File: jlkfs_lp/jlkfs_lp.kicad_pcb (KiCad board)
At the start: 2 copper layers, 139 x 121.8 mm, 38 parts, among them J0 USB_C_Receptacle_PowerOnly_6P, SW0 SWITCH, SW1 SWITCH, SW10 SWITCH, SW11 SWITCH, SW12 SWITCH, SW13 SWITCH, SW14 SWITCH, SW15 SWITCH, SW16 SWITCH, SW17 SWITCH, SW18 SWITCH, SW19 SWITCH, SW2 SWITCH, SW20 SWITCH, SW21 SWITCH, SW22 SWITCH, SW23 SWITCH, SW24 SWITCH, SW25 SWITCH, SW26 SWITCH, SW27 SWITCH, SW28 SWITCH, SW3 SWITCH, SW4 SWITCH, SW5 SWITCH, SW6 SWITCH, SW7 SWITCH, SW8 SWITCH, SW9 SWITCH, U0 RP2040

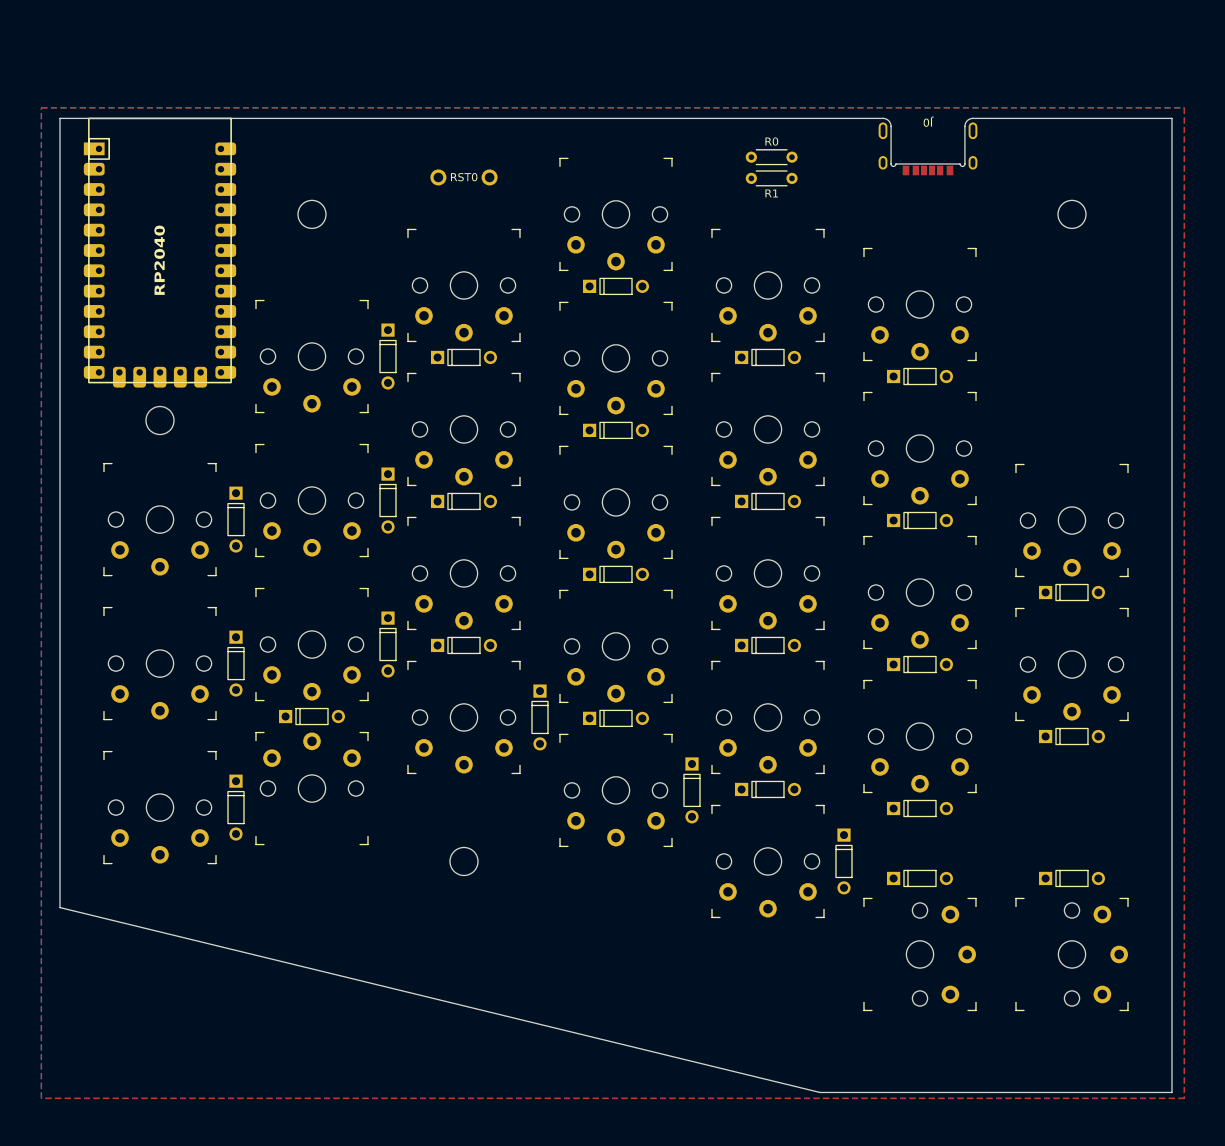
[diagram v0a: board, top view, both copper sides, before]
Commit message: Updates to jlkfs_lp
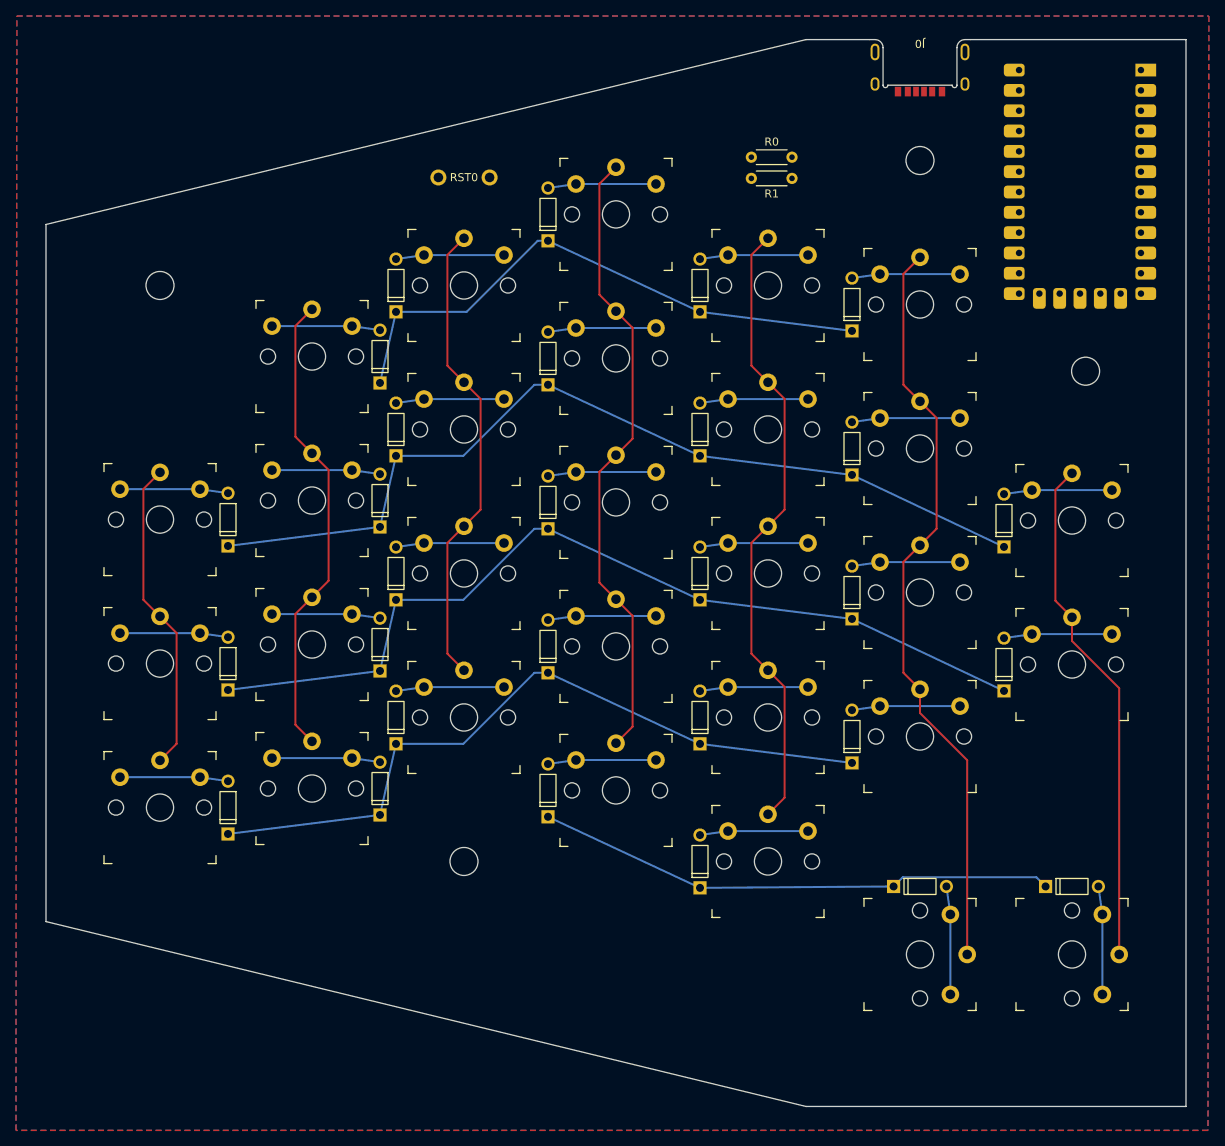
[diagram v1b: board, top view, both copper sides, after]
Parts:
- SW0: renamed from SW3; footprint footprints:kailh_choc_dual_with_side_diode -> footprints:kailh_choc_dual_with_diode; moved to F.Cu
- SW1: renamed from SW7; moved to B.Cu
- SW10: renamed from SW22; moved to B.Cu
- SW11: renamed from SW26; moved to B.Cu
- SW12: renamed from SW1; footprint footprints:kailh_choc_dual_with_side_diode -> footprints:kailh_choc_dual_with_diode; moved to F.Cu
- SW13: renamed from SW5; footprint footprints:kailh_choc_dual_with_side_diode -> footprints:kailh_choc_dual_with_diode; moved to F.Cu
- SW14: renamed from SW9; moved to B.Cu
- SW15: renamed from SW13; moved to B.Cu
- SW16: renamed from SW18; moved to B.Cu
- SW17: renamed from SW23; moved to B.Cu
- SW18: renamed from SW27; moved to B.Cu
- SW19: renamed from SW2; footprint footprints:kailh_choc_dual_with_side_diode -> footprints:kailh_choc_dual_with_diode; moved to F.Cu
- SW2: renamed from SW11; moved to B.Cu
- SW20: renamed from SW6; moved to F.Cu
- SW21: renamed from SW10; footprint footprints:kailh_choc_dual_with_side_diode -> footprints:kailh_choc_dual_with_diode
- SW22: renamed from SW14; moved to B.Cu
- SW23: renamed from SW19; moved to B.Cu
- SW24, U0: moved to B.Cu
- SW25: renamed from SW15; footprint footprints:kailh_choc_dual_with_side_diode -> footprints:kailh_choc_dual_with_diode
- SW26: renamed from SW20; footprint footprints:kailh_choc_dual_with_side_diode -> footprints:kailh_choc_dual_with_diode
- SW27: renamed from SW25; footprint footprints:kailh_choc_dual_with_side_diode -> footprints:kailh_choc_dual_with_diode_15
- SW28: footprint footprints:kailh_choc_dual_with_side_diode -> footprints:kailh_choc_dual_with_diode_15
- SW3: renamed from SW16; moved to B.Cu
- SW4: renamed from SW21; moved to B.Cu
- SW5: renamed from SW0; footprint footprints:kailh_choc_dual_with_side_diode -> footprints:kailh_choc_dual_with_diode; moved to F.Cu
- SW6: renamed from SW4; footprint footprints:kailh_choc_dual_with_side_diode -> footprints:kailh_choc_dual_with_diode; moved to F.Cu
- SW7: renamed from SW8; moved to B.Cu
- SW8: renamed from SW12; moved to B.Cu
- SW9: renamed from SW17; moved to B.Cu
- moved U0 115.4 mm to (206.0, 18.6)
- moved H1 76.3 mm to (186.0, 33.8)
- moved H0 19.7 mm to (206.7, 60.1)
- moved H3 16.9 mm to (91.0, 49.4)
- moved J0 9.90 mm to (186.0, 18.6)
- turned SW20 to 0 degrees
- turned SW21 to 180 degrees
- turned SW25 to 180 degrees
- turned SW26 to 180 degrees
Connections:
- SW10 pad 2: Net-(SW22-A) (its old number) -> Net-(SW10-A)
- SW11 pad 1: /COL0 -> Net-(SW10-A)
- SW11 pad 3: /ROW2 -> /ROW1
- SW18 pad 3: /ROW3 -> /ROW2
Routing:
- net /ROW2: track 0.00 -> 112.1 mm
- net /ROW1: track 0.00 -> 112.1 mm
- net /COL1: track 0.00 -> 94.7 mm
- net /ROW3: track 0.00 -> 91.1 mm
- net /COL2: track 0.00 -> 78.9 mm
- net /COL3: track 0.00 -> 78.9 mm
- net /ROW0: track 0.00 -> 71.9 mm
- net /ROW4: track 0.00 -> 65.1 mm
- net /COL0: track 0.00 -> 64.3 mm
- net /COL5: track 0.00 -> 59.2 mm
- net /COL4: track 0.00 -> 59.2 mm
- net /COL6: track 0.00 -> 39.4 mm
- net Net-(SW9-A): track 0.00 -> 13.5 mm
- net Net-(SW8-A): track 0.00 -> 13.5 mm
- net Net-(SW7-A): track 0.00 -> 13.5 mm
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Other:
- board size 139 x 121.8 mm -> 142.5 x 133.4 mm
